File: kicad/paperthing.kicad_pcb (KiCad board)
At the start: 2 copper layers, 39.3 x 63.4 mm, 20 parts, among them J1 USB_B_Micro, Q1 S8050_J3Y, Q2 PMBT2222AYS, U1 ADXL345BCCZ-RL7, U2 CP2102-GMR_NRND, U3 BL8565, U4 ESP32-S2-WROVER

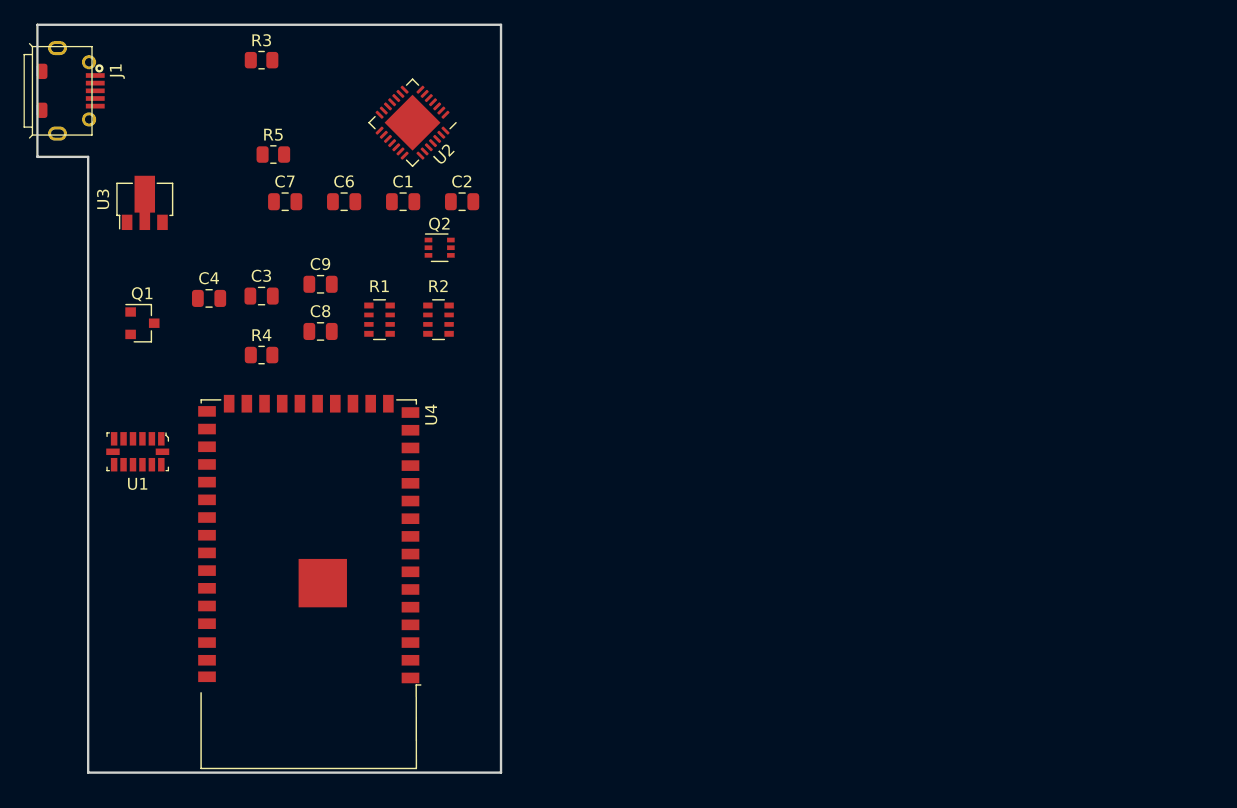
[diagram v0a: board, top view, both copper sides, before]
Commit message: Update paperthing.kicad_pcb
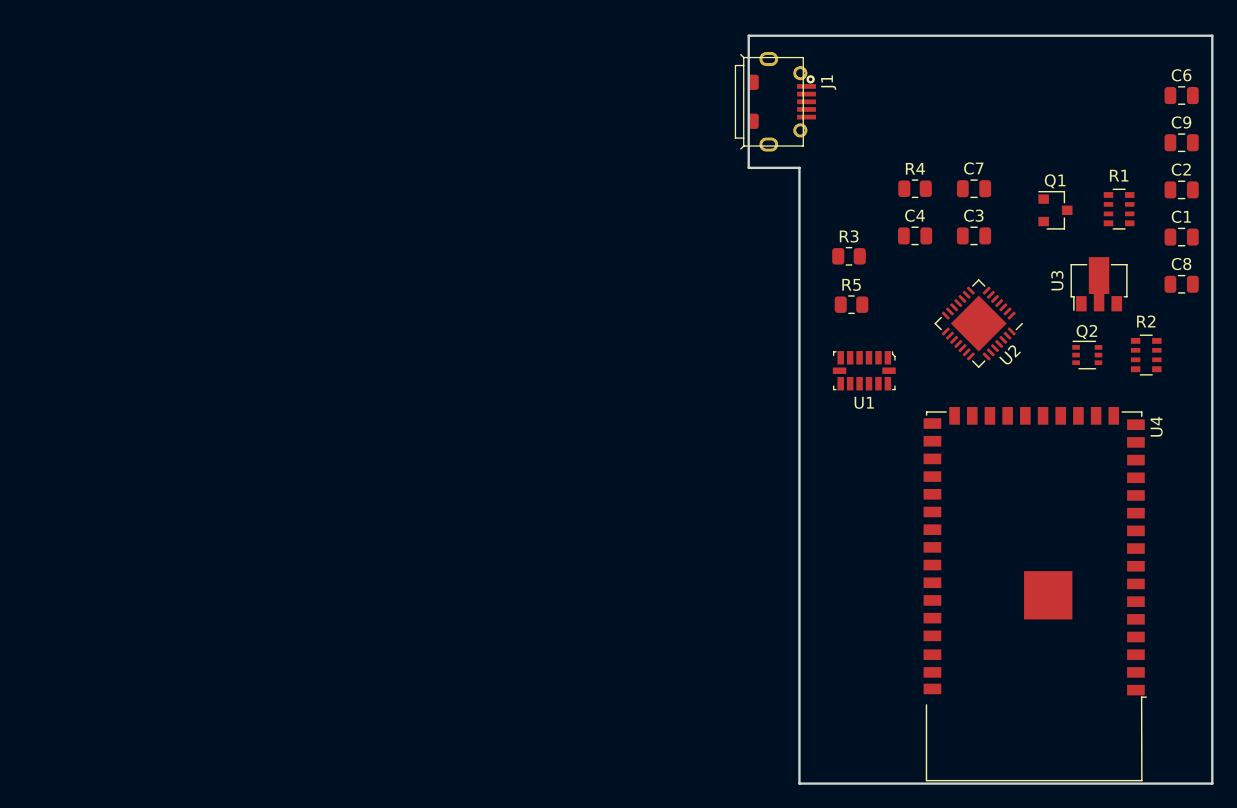
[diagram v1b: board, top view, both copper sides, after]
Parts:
- moved U3 81.2 mm to (150.0, 102.0)
- moved Q1 78.0 mm to (146.3, 95.7)
- moved C9 74.0 mm to (157.0, 90.0)
- moved C8 73.1 mm to (157.0, 102.0)
- moved C6 71.6 mm to (157.0, 86.0)
- moved C1 66.1 mm to (157.0, 98.0)
- moved R1 63.4 mm to (151.7, 95.6)
- moved U1 62.0 mm to (130.1, 109.3)
- moved U4 61.5 mm to (144.5, 124.6)
- moved C2 61.0 mm to (157.0, 94.0)
- moved C3 60.6 mm to (139.4, 97.9)
- moved J1 60.3 mm to (125.2, 86.5)
- moved C4 60.1 mm to (134.4, 97.9)
- moved R2 60.1 mm to (154.0, 108.0)
- moved C7 58.4 mm to (139.4, 93.9)
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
